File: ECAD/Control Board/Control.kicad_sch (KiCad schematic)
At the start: 18 parts

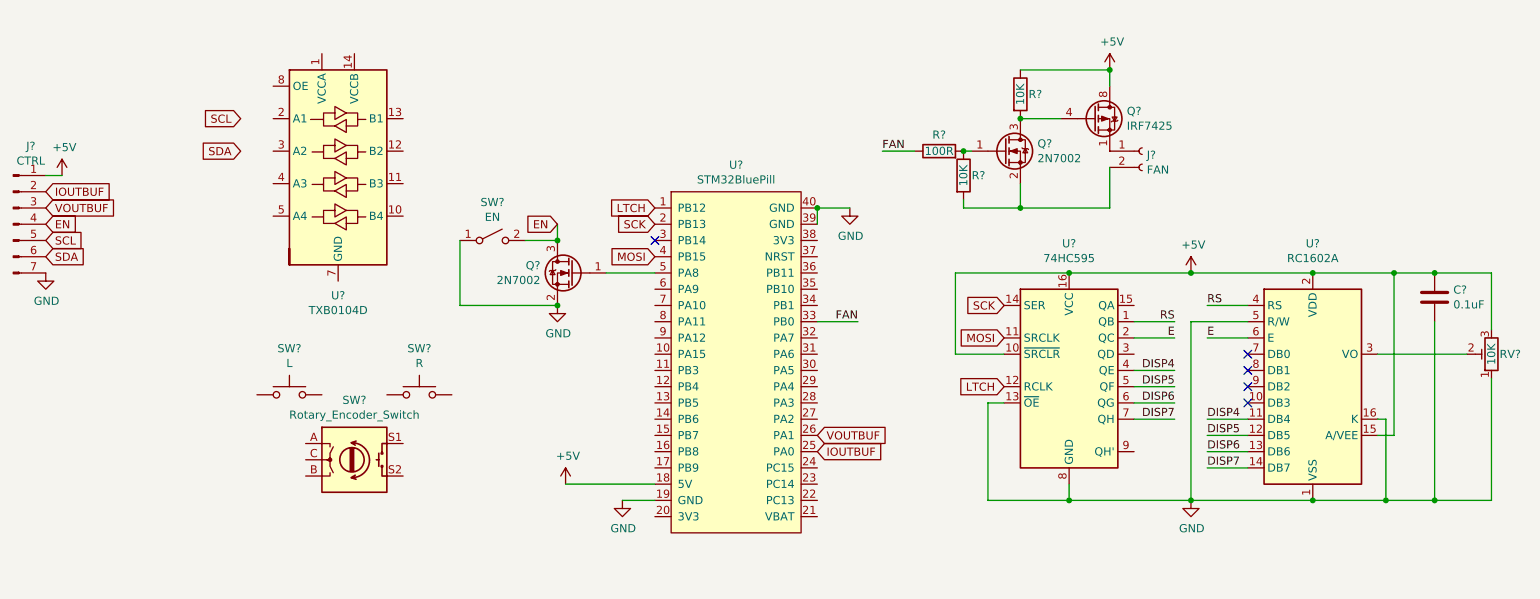
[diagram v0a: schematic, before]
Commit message: havent forgetten about control I swear
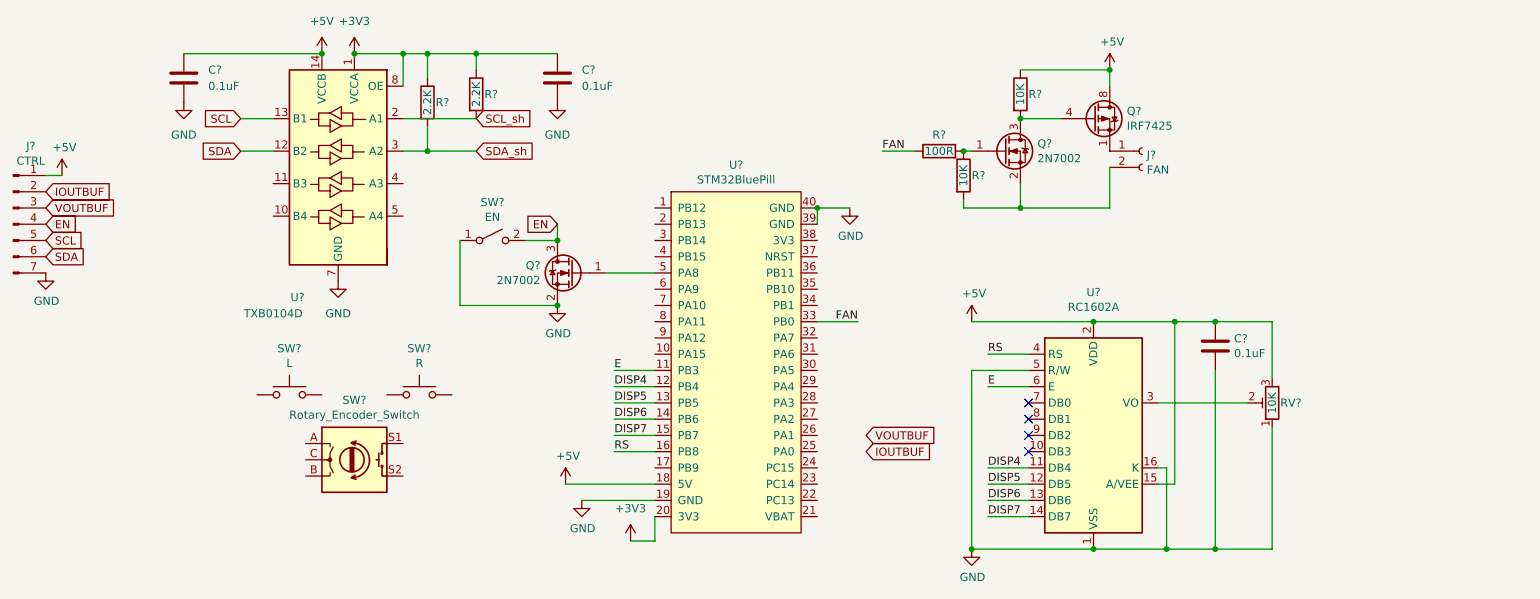
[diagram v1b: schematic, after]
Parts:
- removed U?: 74HC595, symbol 74xx:74HC595
- added C? (x2): 0.1uF, symbol Device:C
- added R? (x2): 2.2K, symbol Device:R
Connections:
- net +5V: now also U?.14 (VCCB), C?.1
- net DISP4: now also U?.12 (PB4)
- net DISP5: now also U?.13 (PB5)
- net DISP6: now also U?.14 (PB6)
- net DISP7: now also U?.15 (PB7)
- net E: now also U?.11 (PB3)
- net GND: now also U?.7 (GND), C?.2, C?.2
- net IOUTBUF: no longer U?.25 (PA0)
- net RS: now also U?.16 (PB8)
- net SCL: now also U?.13 (B1)
- net SDA: now also U?.12 (B2)
- net VOUTBUF: no longer U?.26 (PA1)
- net +3V3: now reaches U?.20 (3V3)
- net +3V3: now also U?.1 (VCCA), U?.8 (OE), C?.1, R?.1, R?.1
- net SCL_sh: now reaches U?.2 (A1)
- net SCL_sh: now also R?.2
- net SDA_sh: now reaches U?.3 (A2)
- net SDA_sh: now also R?.2
- net LTCH: no longer names the net of U?.1 (PB12)
- net MOSI: no longer names the net of U?.4 (PB15)
- net SCK: no longer names the net of U?.2 (PB13)
- no-connect marks 5 -> 4
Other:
- moved on the sheet: C?, RV?, U?
